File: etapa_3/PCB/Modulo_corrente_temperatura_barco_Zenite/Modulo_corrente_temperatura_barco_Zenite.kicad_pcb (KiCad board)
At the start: 2 copper layers, 60 x 150 mm, 11 parts, among them U2 LM7805, U3 TLV9004IDR, U4 MCP2515-xSO, U5 MCP2551-I-SN, Y1 16MHz

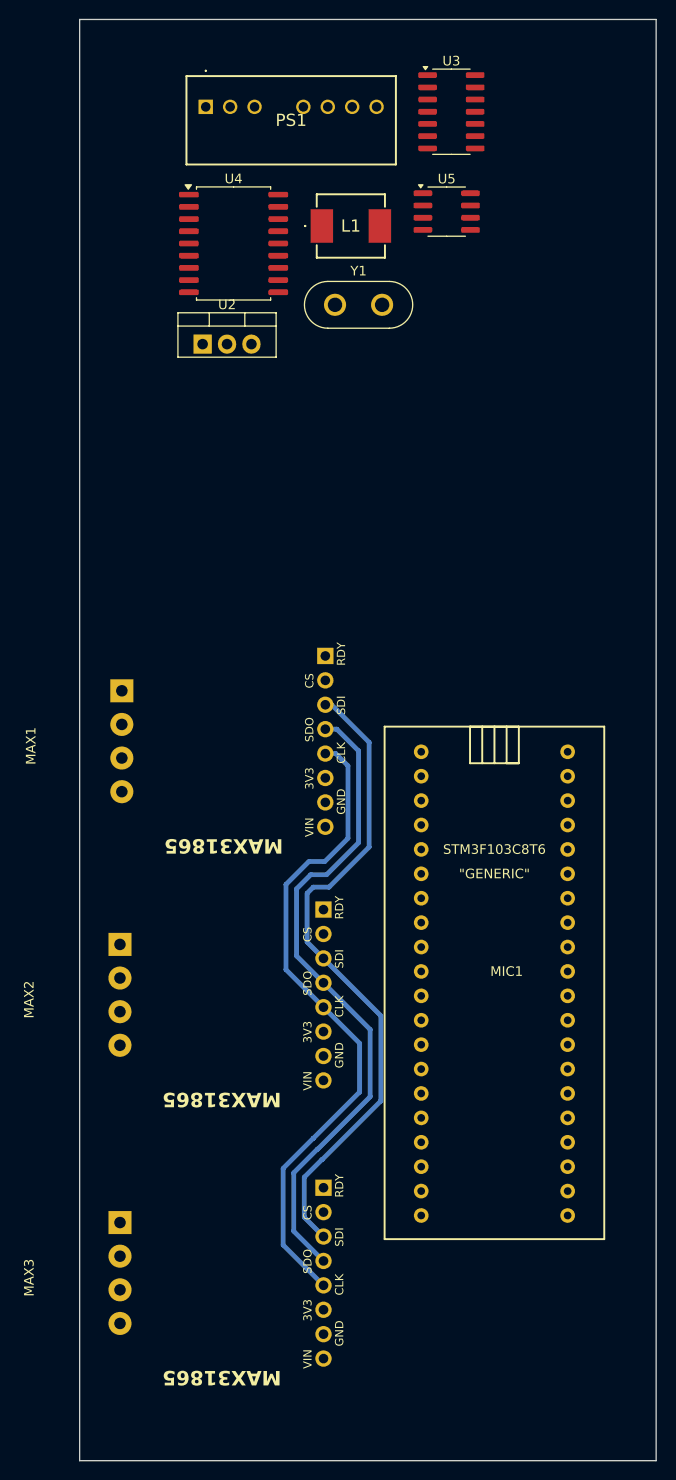
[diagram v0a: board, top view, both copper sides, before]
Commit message: PCB layout V1 added - DRC review nedded
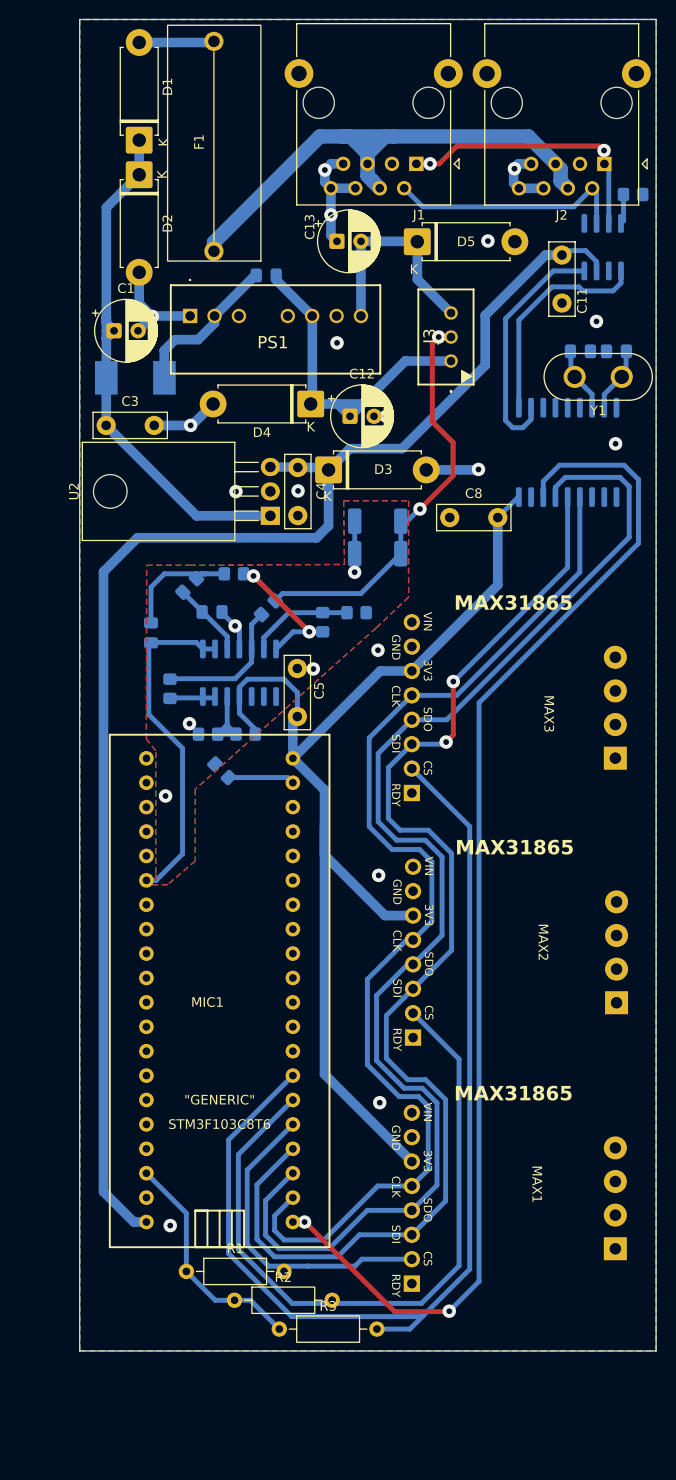
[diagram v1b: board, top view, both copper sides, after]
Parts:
- added C1: 10uF, Capacitor_THT:CP_Radial_D6.3mm_P2.50mm, F.Cu at (84.9, 55.4)
- added C10: 22pF, Capacitor_SMD:C_0805_2012Metric_Pad1.18x1.45mm_HandSolder, B.Cu at (137.2, 57.6)
- added C11: 100nF, Capacitor_THT:C_Disc_D7.5mm_W2.5mm_P5.00mm, F.Cu at (131.5, 47.5)
- added C12: 100uF, Capacitor_THT:CP_Radial_D6.3mm_P2.50mm, F.Cu at (109.4, 64.3)
- added C13: 100uF, Capacitor_THT:CP_Radial_D6.3mm_P2.50mm, F.Cu at (108.1, 46.1)
- added C2: 470pF, Capacitor_SMD:C_0805_2012Metric_Pad1.18x1.45mm_HandSolder, B.Cu at (100.7, 49.7)
- added C3: 220nF, Capacitor_THT:C_Disc_D7.5mm_W2.5mm_P5.00mm, F.Cu at (84.1, 65.3)
- added C4: 100nF, Capacitor_THT:C_Disc_D7.5mm_W2.5mm_P5.00mm, F.Cu at (104.0, 69.7)
- added C5: 100nF, Capacitor_THT:C_Disc_D7.5mm_W2.5mm_P5.00mm, F.Cu at (104.0, 95.6)
- added C6: 470pF, Capacitor_SMD:C_0805_2012Metric_Pad1.18x1.45mm_HandSolder, B.Cu at (95.1, 84.7)
- added C7: 1nF, Capacitor_SMD:C_0805_2012Metric_Pad1.18x1.45mm_HandSolder, B.Cu at (88.7, 86.9)
- added C8: 100nF, Capacitor_THT:C_Disc_D7.5mm_W2.5mm_P5.00mm, F.Cu at (119.8, 74.9)
- added C9: 22pF, Capacitor_SMD:C_0805_2012Metric_Pad1.18x1.45mm_HandSolder, B.Cu at (133.4, 57.6)
- added D1: D, Diode_THT:D_5W_P10.16mm_Horizontal, F.Cu at (87.5, 35.6)
- added D2: D_Zener, Diode_THT:D_5W_P10.16mm_Horizontal, F.Cu at (87.5, 39.2)
- added D3: D_Zener, Diode_THT:D_5W_P10.16mm_Horizontal, F.Cu at (107.2, 69.9)
- added D4: D_Zener, Diode_THT:D_5W_P10.16mm_Horizontal, F.Cu at (105.3, 63.0)
- added D5: D_Zener, Diode_THT:D_5W_P10.16mm_Horizontal, F.Cu at (116.4, 46.1)
- added F1: Fuse, pi-III-lib:fuse_holder, F.Cu at (95.3, 41.6)
- added J1: RJ45_Shielded, Connector_RJ:RJ45_Ninigi_GE, F.Cu at (116.3, 38.0)
- added J2: RJ45_Shielded, Connector_RJ:RJ45_Ninigi_GE, F.Cu at (135.9, 38.1)
- added J3: Conn_01x03, pi-III-lib:B3BXHALFSN, F.Cu at (120.0, 58.6)
- added R1: 100k, Resistor_THT:R_Axial_DIN0207_L6.3mm_D2.5mm_P10.16mm_Horizontal, F.Cu at (92.4, 153.3)
- added R10: 100k, Resistor_SMD:R_0805_2012Metric_Pad1.20x1.40mm_HandSolder, B.Cu at (110.1, 84.8)
- added R11: 10k, Resistor_SMD:R_0805_2012Metric_Pad1.20x1.40mm_HandSolder, B.Cu at (97.4, 80.7)
- added R12: 4k7, Resistor_SMD:R_0805_2012Metric_Pad1.20x1.40mm_HandSolder, B.Cu at (92.8, 81.9)
- added R13: 4k7, Resistor_SMD:R_0805_2012Metric_Pad1.20x1.40mm_HandSolder, B.Cu at (138.9, 41.2)
- added R14: 33, Resistor_SMD:R_2010_5025Metric_Pad1.40x2.65mm_HandSolder, B.Cu at (112.3, 78.6)
- added R15: 0R, Resistor_SMD:R_0805_2012Metric_Pad1.20x1.40mm_HandSolder, B.Cu at (96.1, 101.2)
- added R2: 100k, Resistor_THT:R_Axial_DIN0207_L6.3mm_D2.5mm_P10.16mm_Horizontal, F.Cu at (97.4, 156.3)
- added R3: 100k, Resistor_THT:R_Axial_DIN0207_L6.3mm_D2.5mm_P10.16mm_Horizontal, F.Cu at (102.1, 159.3)
- added R4: 100k, Resistor_SMD:R_0805_2012Metric_Pad1.20x1.40mm_HandSolder, B.Cu at (98.6, 97.4)
- added R5: 100k, Resistor_SMD:R_0805_2012Metric_Pad1.20x1.40mm_HandSolder, B.Cu at (94.7, 97.4)
- added R6: 100k, Resistor_SMD:R_0805_2012Metric_Pad1.20x1.40mm_HandSolder, B.Cu at (90.7, 92.7)
- added R7: 100k, Resistor_SMD:R_0805_2012Metric_Pad1.20x1.40mm_HandSolder, B.Cu at (100.9, 84.2)
- added R8: 33, Resistor_SMD:R_2010_5025Metric_Pad1.40x2.65mm_HandSolder, B.Cu at (112.3, 75.2)
- added R9: 100k, Resistor_SMD:R_0805_2012Metric_Pad1.20x1.40mm_HandSolder, B.Cu at (106.6, 85.8)
- L1, U4, U5: moved to B.Cu
- U2: footprint Package_TO_SOT_THT:TO-220-3_Vertical -> Package_TO_SOT_THT:TO-220-3_Horizontal_TabDown
- U3: value TLV9004IDR -> TLV9004; moved to B.Cu
- moved MAX3 100.0 mm to (149.4, 91.7), turned to -90 degrees
- moved MAX1 86.8 mm to (149.4, 142.8), turned to -90 degrees
- moved MAX2 77.1 mm to (149.6, 117.2), turned to -90 degrees
- moved U3 62.4 mm to (97.9, 91.0), turned to 90 degrees
- moved U4 41.0 mm to (132.1, 68.1), turned to -90 degrees
- moved Y1 30.8 mm to (137.7, 60.2), turned to 180 degrees
- moved MIC1 29.2 mm to (95.9, 126.6), turned to 180 degrees
- moved L1 27.4 mm to (87.1, 60.3)
- moved PS1 21.8 mm to (92.8, 53.9)
- moved U2 19.2 mm to (101.2, 74.7), turned to 90 degrees
- moved U5 16.7 mm to (135.7, 46.7), turned to 90 degrees
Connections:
- MAX1 pad 2: Net-(MAX1-CS) -> A8
- MAX1 pad 3: MOSI3 -> MOSI2
- MAX1 pad 4: MISO3 -> MISO2
- MAX1 pad 5: SCK3 -> SCK2
- MAX2 pad 2: Net-(MAX2-CS) -> A9
- MAX2 pad 3: MOSI3 -> MOSI2
- MAX2 pad 4: MISO3 -> MISO2
- MAX2 pad 5: SCK3 -> SCK2
- MAX3 pad 2: Net-(MAX3-CS) -> A10
- MAX3 pad 3: MOSI3 -> MOSI2
- MAX3 pad 4: MISO3 -> MISO2
- MAX3 pad 5: SCK3 -> SCK2
- MIC1 pad 18: 5V -> unconnected-(MIC1-5V-Pad18)
- MIC1 pad 5: unconnected-(MIC1-A8-Pad5) -> A8
- MIC1 pad 6: unconnected-(MIC1-A9-Pad6) -> A9
- MIC1 pad 7: unconnected-(MIC1-A10-Pad7) -> A10
- U3 pad 1: Net-(U3A--) -> (no net)
- U3 pad 11: GND -> AGND
- U3 pad 2: Net-(U3A--) -> (no net)
- U3 pad 3: Net-(U3A-+) -> (no net)
- U3 pad 5: (no net) -> Net-(U3B-+)
- U3 pad 6: (no net) -> Net-(U3B--)
- U3 pad 7: (no net) -> Net-(U3B--)
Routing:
- net 5V: track 0.00 -> 149.5 mm
- net 3V3: track 0.00 -> 144.7 mm
- net MISO2: track 0.00 -> 135.3 mm
- net NSS2: track 0.00 -> 127.7 mm, vias 0 -> 2
- net MOSI2: track 0.00 -> 127.6 mm, vias 0 -> 2
- net SCK2: track 0.00 -> 116.8 mm
- net A10: track 0.00 -> 111.0 mm
- net A9: track 0.00 -> 73.1 mm
- net MISO3: track 68.9 -> 0.00 mm
- net SCK3: track 68.8 -> 0.00 mm
- net MOSI3: track 68.6 -> 0.00 mm
- net CAN_18V: track 0.00 -> 56.4 mm
- net CAN_18V_p: track 0.00 -> 55.0 mm
- net GND: track 0.00 -> 51.8 mm, vias 0 -> 17
- net I_signal: track 0.00 -> 43.5 mm, vias 0 -> 2
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- added copper zone on B.Cu, net AGND
- added copper zone on F.Cu, net AGND
- added copper zone on B.Cu, net GND
- added copper zone on F.Cu, net GND
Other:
- board size 60 x 150 mm -> 60 x 138.6 mm
